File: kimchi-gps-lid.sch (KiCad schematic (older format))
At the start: 22 parts, among them J1 DF40HC(3.5)-60DS, J2 DF40HC(3.5)-60DS, Q1 DTC143ZEBTL, Q2 DTC143ZEBTL, U1 24C32, U2 L80RE-M37, U3 TXS0104ED

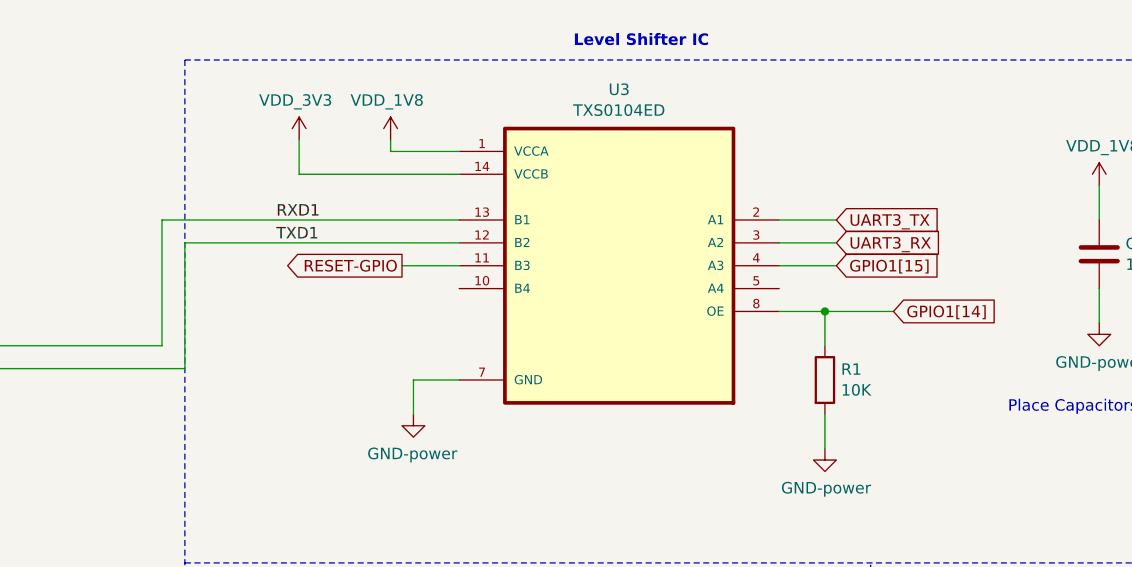
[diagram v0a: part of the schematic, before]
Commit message: Update layout and routing
Signed-off-by: Michael Welling <mwelling@ieee.org>
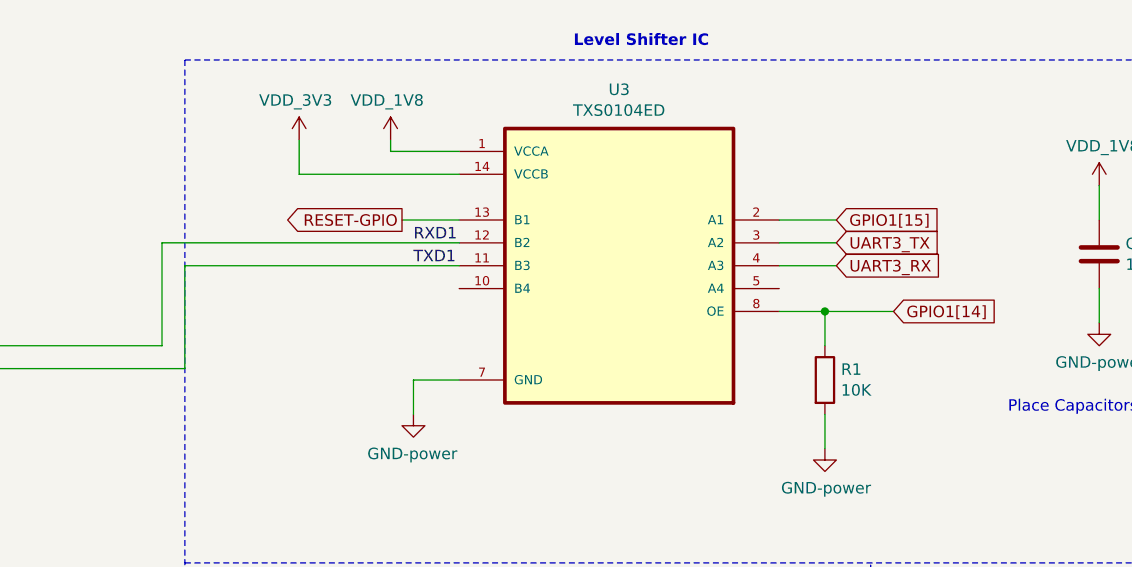
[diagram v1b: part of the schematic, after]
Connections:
- net GPIO1[15]: now also U3.2 (A1); no longer U3.4 (A3)
- net RESET-GPIO: now also U3.13 (B1); no longer U3.11 (B3)
- net RXD1: now also U3.12 (B2); no longer U3.13 (B1)
- net TXD1: now also U3.11 (B3); no longer U3.12 (B2)
- net UART3_RX: now also U3.4 (A3); no longer U3.3 (A2)
- net UART3_TX: now also U3.3 (A2); no longer U3.2 (A1)
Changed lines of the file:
@@
 	-1   0    0    -1
 $EndComp
-Wire Wire Line
-	8450 5500 7150 5500
-Wire Wire Line
-	7250 5600 8450 5600
-Text GLabel 10100 5600 2    50   Input ~ 0
+Text GLabel 10100 5700 2    50   Input ~ 0
 UART3_RX
-Text Label 7650 5500 0    50   ~ 0
+Text Label 8250 5600 0    50   ~ 0
 RXD1
-Text Label 7650 5600 0    50   ~ 0
+Text Label 8250 5700 0    50   ~ 0
 TXD1
 $Comp
@@
 	1    0    0    -1
 $EndComp
-Text GLabel 8200 5700 0    50   Output ~ 0
+Text GLabel 8200 5500 0    50   Output ~ 0
 RESET-GPIO
 Wire Wire Line
-	8450 5700 8200 5700
+	8450 5500 8200 5500
 Text GLabel 5900 5650 2    50   Input ~ 0
 RESET
@@
 Text Notes 8950 4750 0    50   ~ 10
 Level Shifter IC
+Text GLabel 10100 5600 2    50   Input ~ 0
+UART3_TX
+Wire Wire Line
+	9850 5500 10100 5500
+Wire Wire Line
+	5700 6150 7250 6150
+Wire Wire Line
+	7150 6050 5700 6050
+Wire Wire Line
+	9850 5600 10100 5600
 Text GLabel 10100 5500 2    50   Input ~ 0
-UART3_TX
-Wire Wire Line
-	9850 5500 10100 5500
-Wire Wire Line
-	5700 6150 7250 6150
-Wire Wire Line
-	7150 6050 5700 6050
-Wire Wire Line
-	7250 6150 7250 5600
-Wire Wire Line
-	7150 5500 7150 6050
-Wire Wire Line
-	9850 5600 10100 5600
-Text GLabel 10100 5700 2    50   Input ~ 0
 GPIO1[15]
 Wire Wire Line
@@
 Text Notes 8000 8950 0    50   ~ 0
 Place 100n near the GPS module\n
+Wire Wire Line
+	7150 5600 7150 6050
+Wire Wire Line
+	7150 5600 8450 5600
+Wire Wire Line
+	7250 6150 7250 5700
+Wire Wire Line
+	7250 5700 8450 5700
 $EndSCHEMATC
